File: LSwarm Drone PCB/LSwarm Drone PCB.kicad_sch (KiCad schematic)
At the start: 130 parts, among them J2 Conn_01x06_Pin, J3 JST / BT2.0 Connector, J4 Conn_01x02_Pin, J5 Conn_01x02_Pin, J6 Conn_01x02_Pin, J7 Conn_01x02_Pin, J8 Conn_01x05_Pin, Q1 AO3400A, Q2 AO3400A, Q3 AO3400A, Q4 AO3400A, Q7 AO3407A, SW1 MSK12C02, SW2 SKRPACE010, SW3 SKRPACE010, SW4 SKRPACE010, SW5 SKRPACE010, U1 LSM6DSRTR, U12 AP2112K-3.3, U3 TPS61023DRLR, U4 SN74LVC1T45DBVR, U5 BMP581, X1 X322512MSB4SI

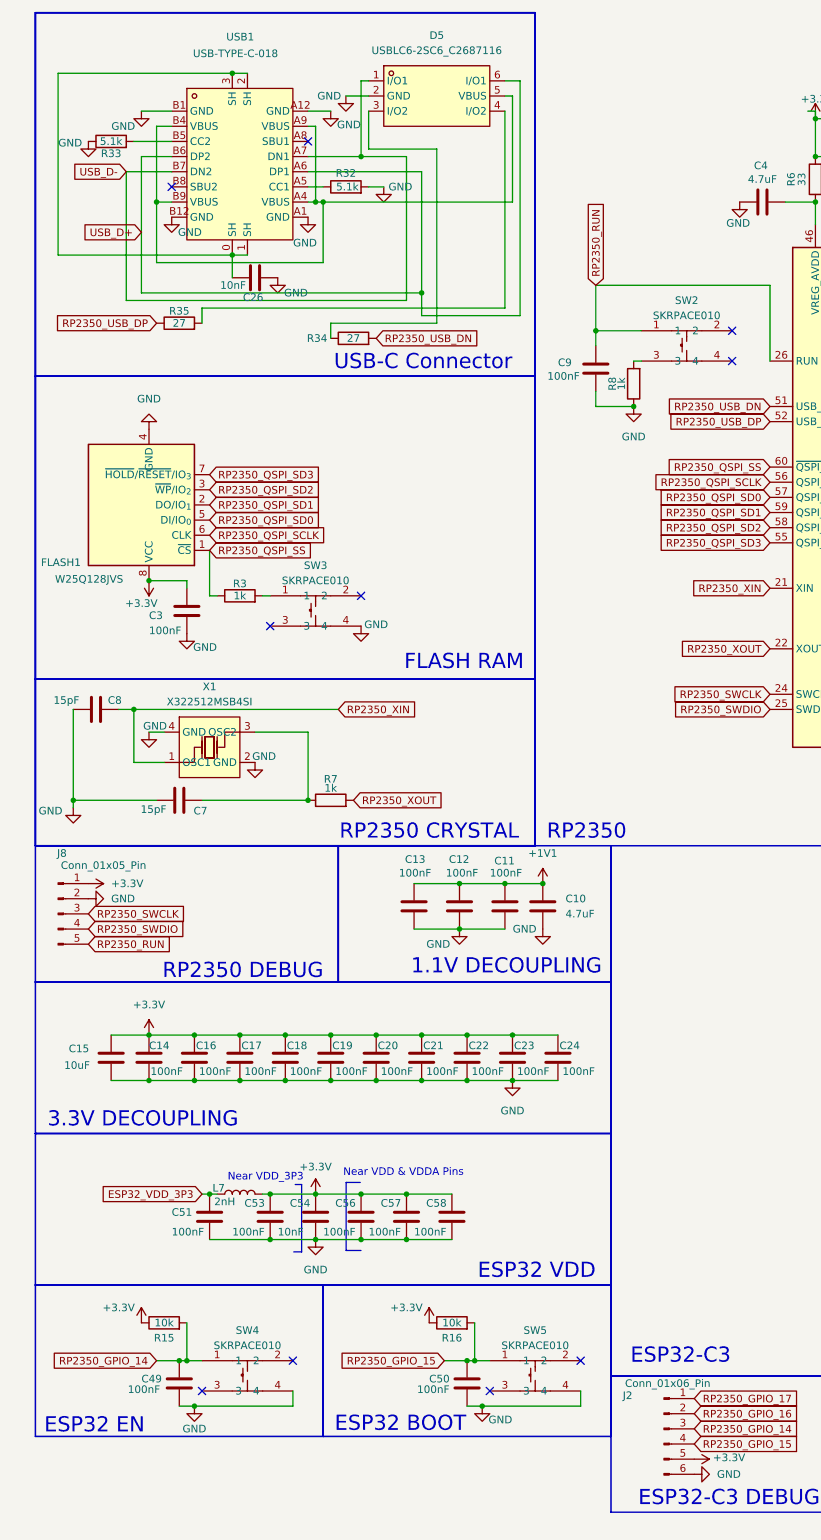
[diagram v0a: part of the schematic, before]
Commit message: sync
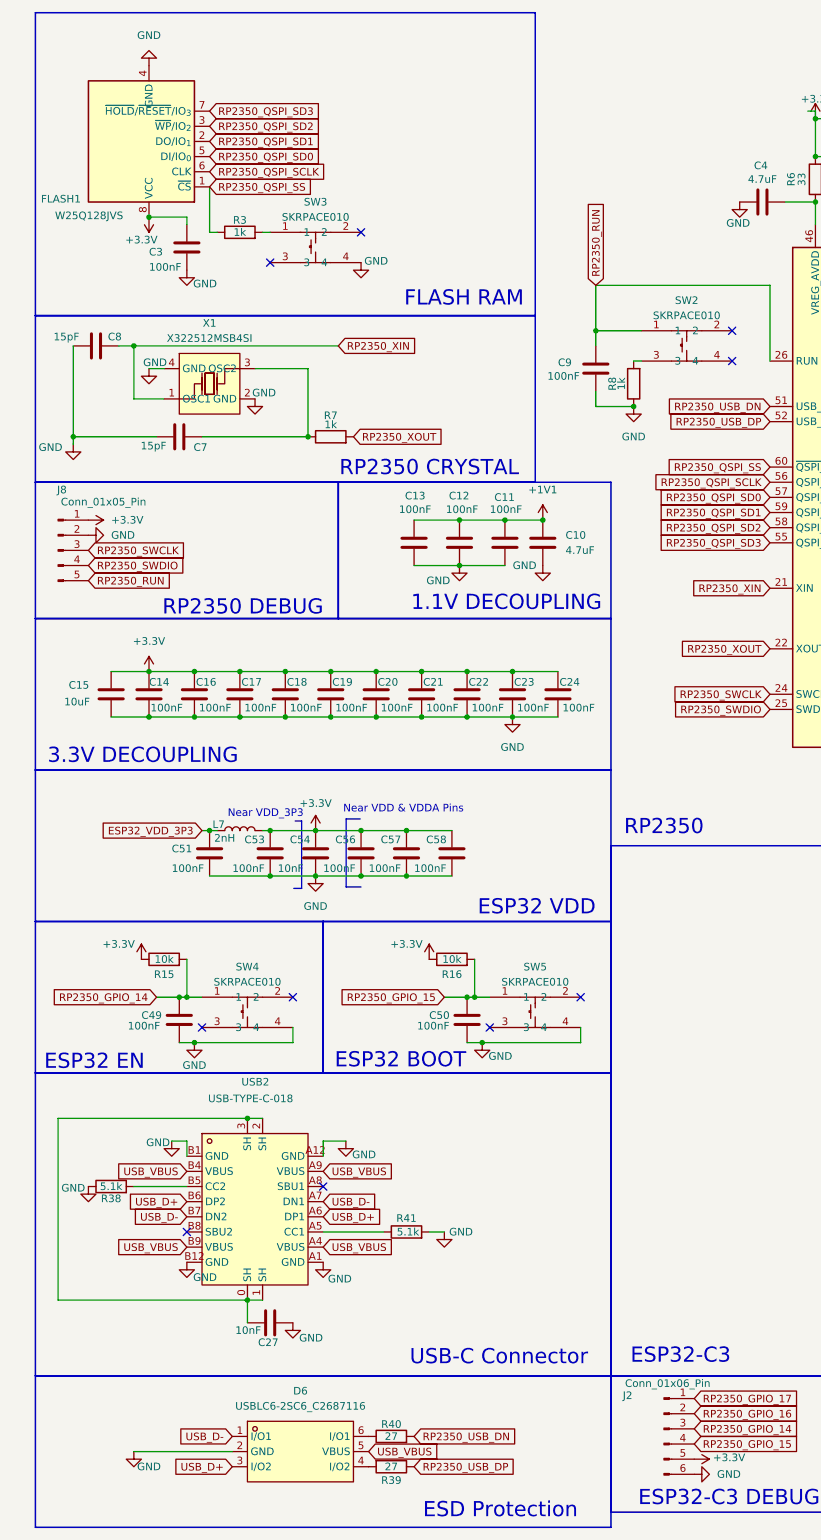
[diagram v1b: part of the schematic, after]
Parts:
- removed C26: 10nF, Capacitor_SMD:C_0603_1608Metric, symbol Device:C
- removed D5: USBLC6-2SC6_C2687116, easyeda2kicad:SOT-23-6_L2.9-W1.6-P0.95-LS2.8-BL, symbol easyeda2kicad:USBLC6-2SC6_C2687116
- removed R32, R33: 5.1k, Resistor_SMD:R_0603_1608Metric, symbol Device:R
- removed R34, R35: 27, Resistor_SMD:R_0603_1608Metric, symbol Device:R
- removed USB1: USB-TYPE-C-018, easyeda2kicad:USB-C_SMD-TYPE-C-31-M-12, symbol easyeda2kicad:USB-TYPE-C-018
- added C27: 10nF, Capacitor_SMD:C_0603_1608Metric, symbol Device:C
- added D6: USBLC6-2SC6_C2687116, easyeda2kicad:SOT-23-6_L2.9-W1.6-P0.95-LS2.8-BL, symbol easyeda2kicad:USBLC6-2SC6_C2687116
- added R38, R41: 5.1k, Resistor_SMD:R_0603_1608Metric, symbol Device:R
- added R39, R40: 27, Resistor_SMD:R_0603_1608Metric, symbol Device:R
- added USB2: USB-TYPE-C-018, easyeda2kicad:USB-C_SMD-TYPE-C-31-M-12, symbol easyeda2kicad:USB-TYPE-C-018
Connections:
- net GND: now also C27.1, D6.2 (GND), R38.1, R41.2, USB2.A1 (GND), USB2.A12 (GND), USB2.B1 (GND), USB2.B12 (GND)
- net RP2350_USB_DN: now also R40.2
- net RP2350_USB_DP: now also R39.1
- net USB_D+: now also D6.3 (I/O2), USB2.A6 (DP1), USB2.B6 (DP2)
- net USB_D-: now also D6.1 (I/O1), USB2.A7 (DN1), USB2.B7 (DN2)
- new net: D6.6 (I/O1), R40.1
- new net: D6.4 (I/O2), R39.2
- new net: R41.1, USB2.A5 (CC1)
- new net: R38.2, USB2.B5 (CC2)
- new net: C27.2, USB2.0 (SH), USB2.1 (SH), USB2.2 (SH), USB2.3 (SH)
- new net USB_VBUS: D6.5 (VBUS), USB2.A4 (VBUS), USB2.A9 (VBUS), USB2.B4 (VBUS), USB2.B9 (VBUS)
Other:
- note added: "ESD Protection"
- moved on the sheet: C10, C11, C12, C13, C14, C15, C16, C17, C18, C19, C20, C21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
